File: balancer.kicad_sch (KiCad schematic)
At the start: 3 parts, among them J1 Conn_01x20, J2 Conn_01x20, J3 Conn_01x04

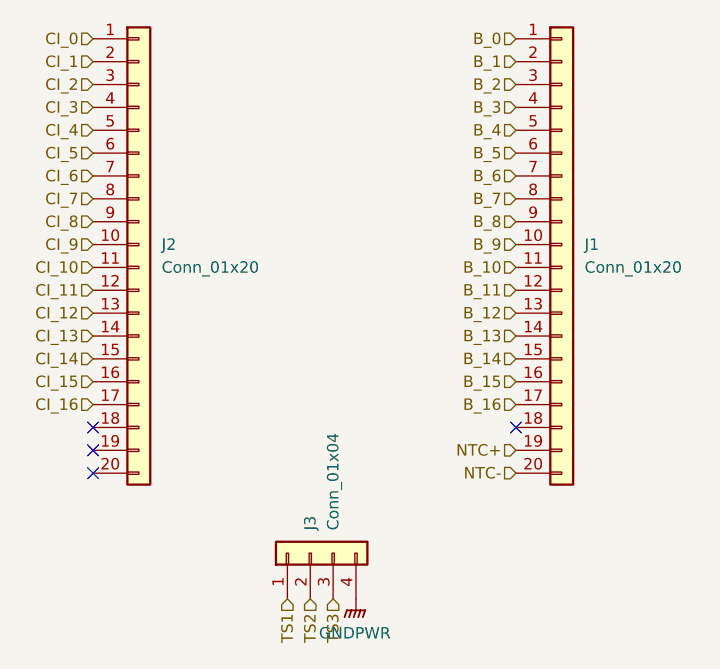
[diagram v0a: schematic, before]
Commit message: BMS DONE IHOPE
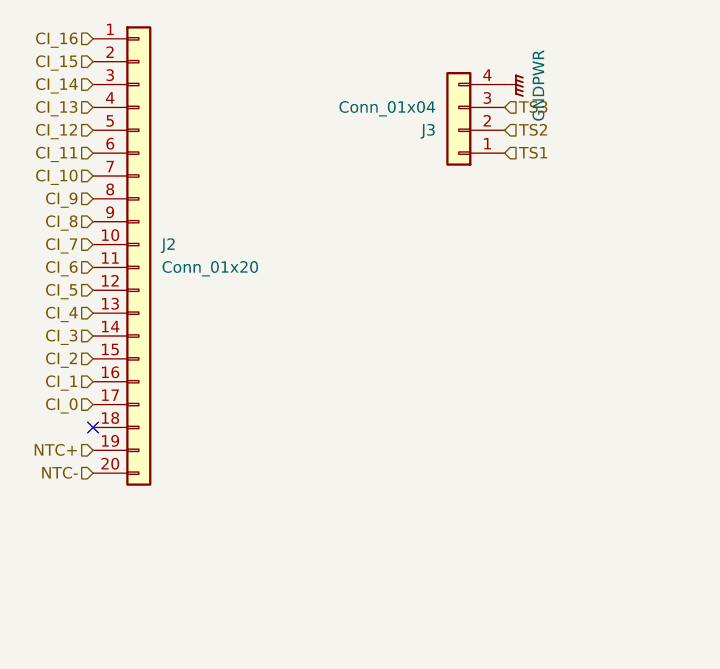
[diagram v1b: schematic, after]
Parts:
- removed J1: Conn_01x20, Connector_PinSocket_2.54mm:PinSocket_1x20_P2.54mm_Vertical_SMD_Pin1Right, symbol Connector_Generic:Conn_01x20
- J2: footprint Connector_PinSocket_2.54mm:PinSocket_1x20_P2.54mm_Horizontal -> Connector_Wago:Wago_734-180_1x20_P3.50mm_Horizontal
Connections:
- net CI_0: now also J2.17 (Pin_17); no longer J2.1 (Pin_1)
- net CI_1: now also J2.16 (Pin_16); no longer J2.2 (Pin_2)
- net CI_10: now also J2.7 (Pin_7); no longer J2.11 (Pin_11)
- net CI_11: now also J2.6 (Pin_6); no longer J2.12 (Pin_12)
- net CI_12: now also J2.5 (Pin_5); no longer J2.13 (Pin_13)
- net CI_13: now also J2.4 (Pin_4); no longer J2.14 (Pin_14)
- net CI_14: now also J2.3 (Pin_3); no longer J2.15 (Pin_15)
- net CI_15: now also J2.2 (Pin_2); no longer J2.16 (Pin_16)
- net CI_16: now also J2.1 (Pin_1); no longer J2.17 (Pin_17)
- net CI_2: now also J2.15 (Pin_15); no longer J2.3 (Pin_3)
- net CI_3: now also J2.14 (Pin_14); no longer J2.4 (Pin_4)
- net CI_4: now also J2.13 (Pin_13); no longer J2.5 (Pin_5)
- net CI_5: now also J2.12 (Pin_12); no longer J2.6 (Pin_6)
- net CI_6: now also J2.11 (Pin_11); no longer J2.7 (Pin_7)
- net CI_7: now also J2.10 (Pin_10); no longer J2.8 (Pin_8)
- net CI_9: now also J2.8 (Pin_8); no longer J2.10 (Pin_10)
- net NTC+: now also J2.19 (Pin_19)
- net NTC-: now also J2.20 (Pin_20)
- no-connect marks 4 -> 1
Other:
- moved on the sheet: J3
